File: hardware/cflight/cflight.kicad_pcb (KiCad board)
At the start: 2 copper layers, 30.5 x 81.3 mm, 13 parts, among them J1 GPS connector, J2 GPRS connector, U1 ESP32-DEVKIT-V1

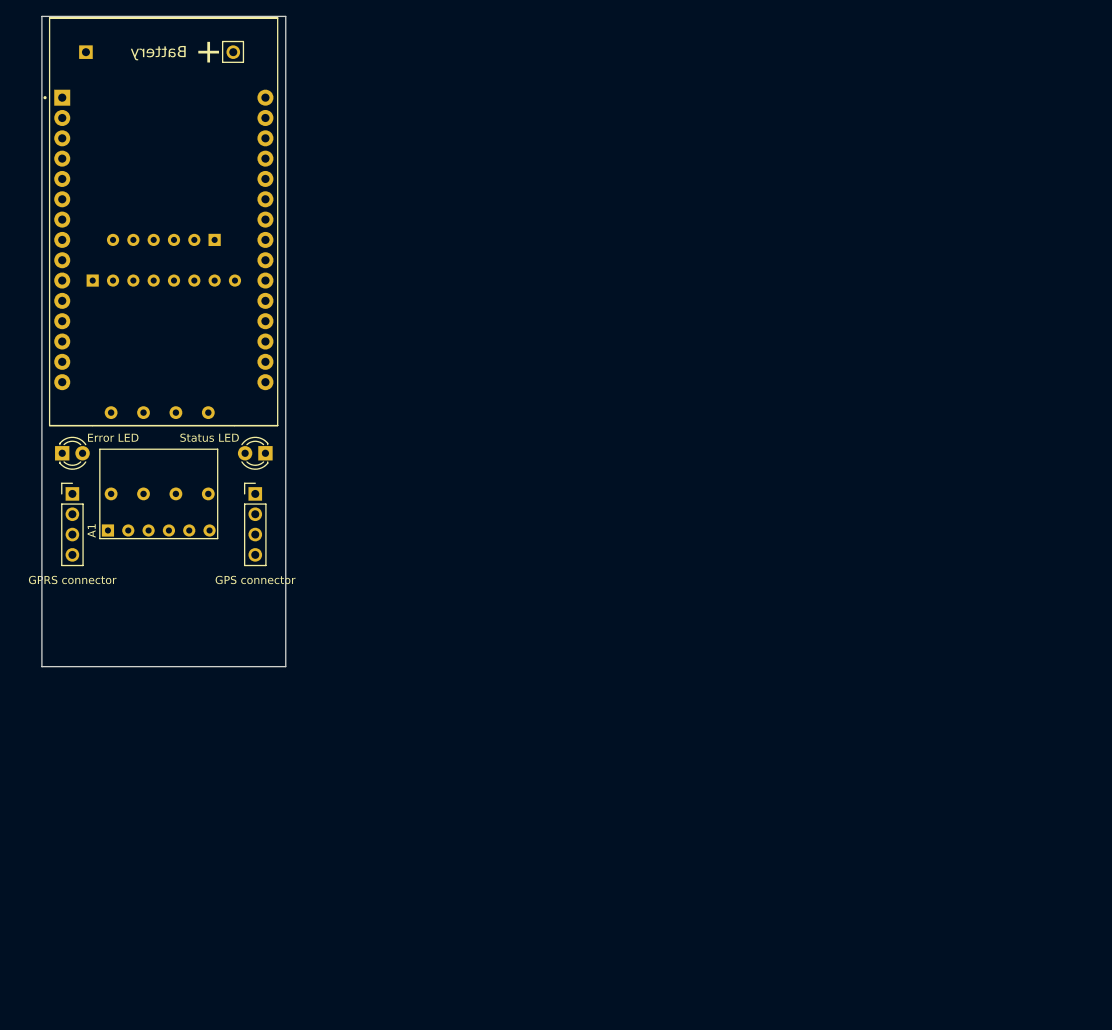
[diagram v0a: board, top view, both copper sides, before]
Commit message: college prog
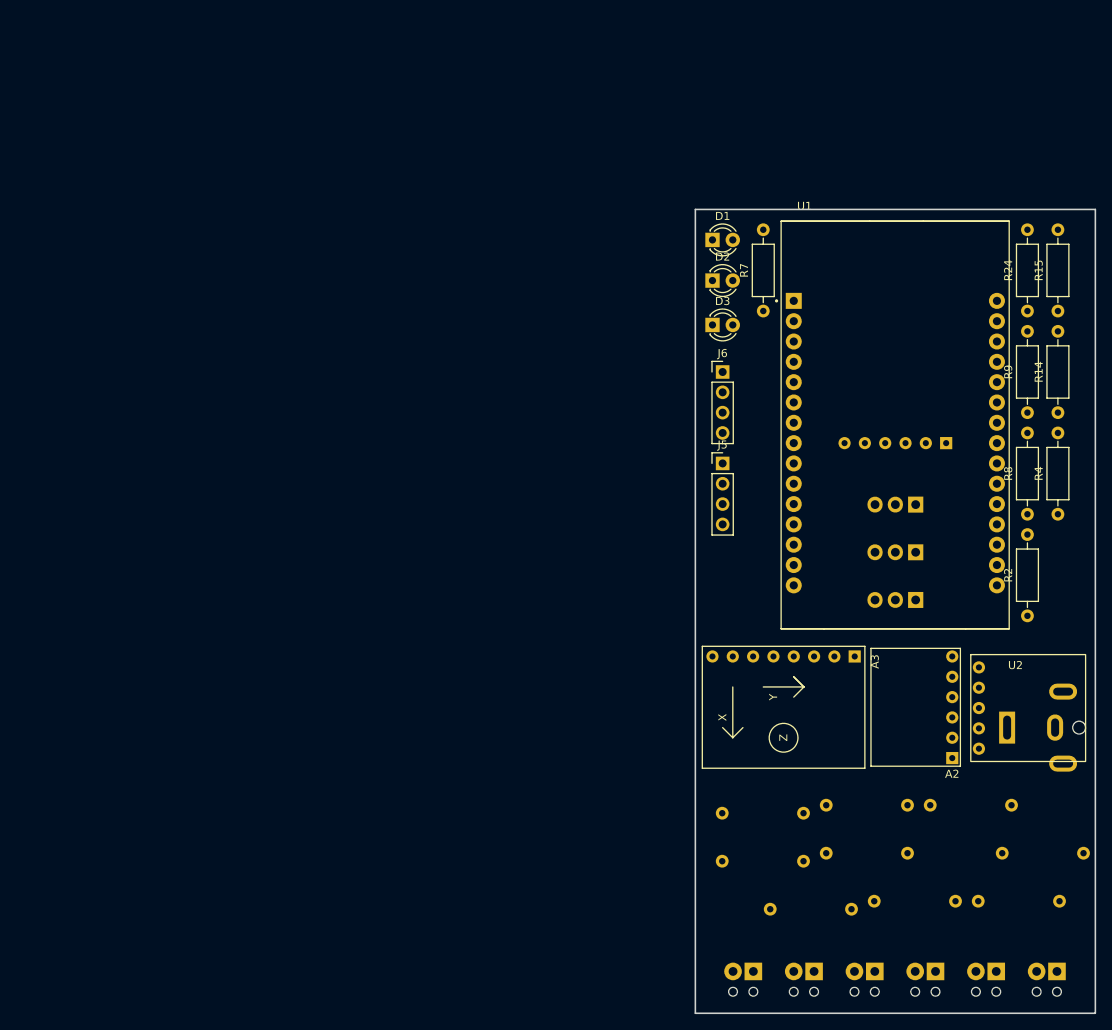
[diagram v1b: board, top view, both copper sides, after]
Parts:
- removed Battery1: Battery_Cell, Connector_PinSocket_2.54mm:PinSocket_1x02_P2.54mm_Vertical
- added D3: Status LED, LED_THT:LED_D3.0mm, F.Cu at (134.6, 64.0)
- added J10: CH_{2}, TerminalBlock_Phoenix:TerminalBlock_Phoenix_MPT-0,5-2-2.54_1x02_P2.54mm_Horizontal, B.Cu at (177.7, 144.8)
- added J3: 3.3v, TerminalBlock_Phoenix:TerminalBlock_Phoenix_MPT-0,5-2-2.54_1x02_P2.54mm_Horizontal, B.Cu at (154.9, 144.8)
- added J4: CH_{1}, TerminalBlock_Phoenix:TerminalBlock_Phoenix_MPT-0,5-2-2.54_1x02_P2.54mm_Horizontal, B.Cu at (162.5, 144.8)
- added J5: GPS connector, Connector_PinHeader_2.54mm:PinHeader_1x04_P2.54mm_Vertical, F.Cu at (135.9, 81.3)
- added J6: GPRS connector, Connector_PinHeader_2.54mm:PinHeader_1x04_P2.54mm_Vertical, F.Cu at (135.9, 69.8)
- added J7: CH_{3}, TerminalBlock_Phoenix:TerminalBlock_Phoenix_MPT-0,5-2-2.54_1x02_P2.54mm_Horizontal, B.Cu at (170.1, 144.8)
- added J8: Barrel_Jack_Switch, Connector_BarrelJack:BarrelJack_CUI_PJ-063AH_Horizontal, B.Cu at (171.4, 114.3)
- added Q1: TIP122, Package_TO_SOT_THT:TO-220-3_Vertical, B.Cu at (160.0, 86.4)
- added Q2: TIP122, Package_TO_SOT_THT:TO-220-3_Vertical, B.Cu at (160.0, 92.4)
- added Q3: TIP122, Package_TO_SOT_THT:TO-220-3_Vertical, B.Cu at (160.0, 98.3)
- added R10: 4k7, Resistor_THT:R_Axial_DIN0207_L6.3mm_D2.5mm_P10.16mm_Horizontal, B.Cu at (172.0, 124.0)
- added R11: 5k, Resistor_THT:R_Axial_DIN0207_L6.3mm_D2.5mm_P10.16mm_Horizontal, B.Cu at (146.0, 131.0)
- added R12: 10k, Resistor_THT:R_Axial_DIN0207_L6.3mm_D2.5mm_P10.16mm_Horizontal, B.Cu at (152.0, 137.0)
- added R13: 4k7, Resistor_THT:R_Axial_DIN0207_L6.3mm_D2.5mm_P10.16mm_Horizontal, B.Cu at (159.0, 124.0)
- added R14: 470, Resistor_THT:R_Axial_DIN0207_L6.3mm_D2.5mm_P10.16mm_Horizontal, F.Cu at (177.8, 74.9)
- added R15: 80, Resistor_THT:R_Axial_DIN0207_L6.3mm_D2.5mm_P10.16mm_Horizontal, F.Cu at (177.8, 62.2)
- added R23: 4k7, Resistor_THT:R_Axial_DIN0207_L6.3mm_D2.5mm_P10.16mm_Horizontal, B.Cu at (159.0, 130.0)
- added R24: 470, Resistor_THT:R_Axial_DIN0207_L6.3mm_D2.5mm_P10.16mm_Horizontal, F.Cu at (174.0, 62.2)
- added R5: 12k, Resistor_THT:R_Axial_DIN0207_L6.3mm_D2.5mm_P10.16mm_Horizontal, B.Cu at (165.0, 136.0)
- added R6: 10k, Resistor_THT:R_Axial_DIN0207_L6.3mm_D2.5mm_P10.16mm_Horizontal, B.Cu at (181.0, 130.0)
- added R7: 80, Resistor_THT:R_Axial_DIN0207_L6.3mm_D2.5mm_P10.16mm_Horizontal, F.Cu at (141.0, 62.2)
- added R8: 470, Resistor_THT:R_Axial_DIN0207_L6.3mm_D2.5mm_P10.16mm_Horizontal, F.Cu at (174.0, 87.6)
- added R9: 50, Resistor_THT:R_Axial_DIN0207_L6.3mm_D2.5mm_P10.16mm_Horizontal, F.Cu at (174.0, 74.9)
- added U2: ~, Modules:GY-271, F.Cu at (166.9, 105.2)
- A1: value BMP280_Module -> SD_Card_Module; footprint Modules:BMP280_Module -> Modules:SD_Card_Module; moved to B.Cu
- A2: value SD_Card_Module -> BMP280_Module; footprint Modules:SD_Card_Module -> Modules:BMP280_Module; moved to F.Cu
- A3: moved to F.Cu
- D1: value Error LED -> Arm LED
- D2: value Status LED -> Error LED
- J1: value GPS connector -> 7.2v; footprint Connector_PinHeader_2.54mm:PinHeader_1x04_P2.54mm_Vertical -> TerminalBlock_Phoenix:TerminalBlock_Phoenix_MPT-0,5-2-2.54_1x02_P2.54mm_Horizontal; moved to B.Cu
- J2: value GPRS connector -> I2C; footprint Connector_PinHeader_2.54mm:PinHeader_1x04_P2.54mm_Vertical -> TerminalBlock_Phoenix:TerminalBlock_Phoenix_MPT-0,5-2-2.54_1x02_P2.54mm_Horizontal; moved to B.Cu
- R1: value 80 -> 10k
- R2: value 50 -> 18k; moved to F.Cu
- R3: value 1800 -> 5k
- R4: value 1200 -> 5k; moved to F.Cu
- moved R1 129.0 mm to (178.0, 136.0), turned to 180 degrees
- moved A2 112.7 mm to (164.6, 118.1), turned to 180 degrees
- moved R2 111.5 mm to (174.0, 100.3)
- moved J2 110.3 mm to (147.3, 144.8), turned to 180 degrees
- moved R4 106.2 mm to (177.8, 87.6)
- moved A3 106.2 mm to (152.4, 105.4)
- moved A1 105.3 mm to (163.8, 78.7)
- moved U1 94.9 mm to (157.5, 76.5)
- moved R3 88.0 mm to (146.0, 125.0), turned to 180 degrees
- moved J1 86.3 mm to (139.7, 144.8), turned to 180 degrees
- moved D1 85.5 mm to (134.6, 53.3)
- moved D2 59.9 mm to (134.6, 58.4), turned to 0 degrees
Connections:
- A1 pad 2: Batt_{gnd} -> SPI_{CS}
- A1 pad 3: SCL -> MOSI
- A1 pad 4: SDA -> SPI_{CLK}
- A1 pad 5: unconnected-(A1-CSB-Pad5) -> MISO
- A1 pad 6: unconnected-(A1-SD0-Pad6) -> Batt_{gnd}
- A2 pad 2: SPI_{CS} -> Batt_{gnd}
- A2 pad 3: MOSI -> SCL
- A2 pad 4: SPI_{CLK} -> SDA
- A2 pad 5: MISO -> unconnected-(A2-CSB-Pad5)
- A2 pad 6: Batt_{gnd} -> unconnected-(A2-SD0-Pad6)
- A3 pad 1: unconnected-(A3-VCC-Pad1) -> +3.3V
- J1 pad 1: +3.3V -> V_{batt}
- J2 pad 1: +3.3V -> SCL
- J2 pad 2: Batt_{gnd} -> SDA
- R1 pad 1: Net-(D1-A) -> CH_{1}^{test}
- R1 pad 2: LED_{status} -> Net-(J4-Pin_2)
- R2 pad 1: Net-(D2-A) -> V_{batt}
- R2 pad 2: LED_{error} -> BATT_{check}
- R3 pad 1: V_{batt} -> Batt_{gnd}
- R3 pad 2: BATT_{check} -> CH_{1}^{test}
- R4 pad 2: BATT_{check} -> CH_{2}^{test}
- U1 pad 19: unconnected-(U1-D34-Pad19) -> CH_{2}^{test}
- U1 pad 20: unconnected-(U1-D35-Pad20) -> CH_{2}^{fire}
- U1 pad 21: unconnected-(U1-D32-Pad21) -> CH_{1}^{fire}
- U1 pad 22: unconnected-(U1-D33-Pad22) -> CH_{1}^{test}
- U1 pad 27: unconnected-(U1-D12-Pad27) -> CH_{3}^{test}
- U1 pad 28: unconnected-(U1-D13-Pad28) -> CH_{3}^{fire}
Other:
- board size 30.5 x 81.3 mm -> 50 x 100.5 mm
- board text removed: "Battery"

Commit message: Continue hardware
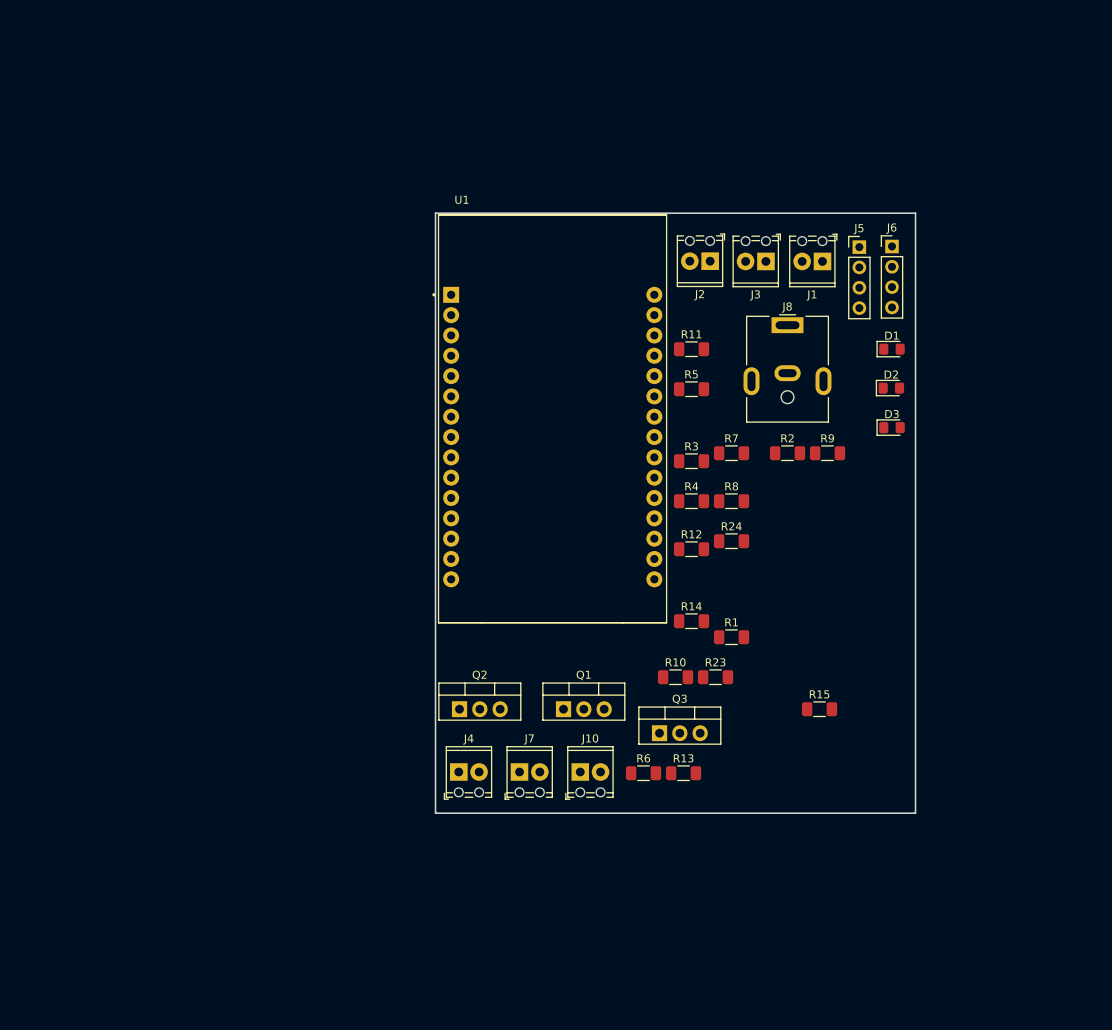
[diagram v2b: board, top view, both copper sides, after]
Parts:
- removed A1: SD_Card_Module, Modules:SD_Card_Module
- removed A2: BMP280_Module, Modules:BMP280_Module
- removed A3: MPU6050, Modules:MPU6050_Module
- removed U2: ~, Modules:GY-271
- D1: value Arm LED -> Armed; footprint LED_THT:LED_D3.0mm -> LED_SMD:LED_0805_2012Metric_Pad1.15x1.40mm_HandSolder
- D2: value Error LED -> Error; footprint LED_THT:LED_D3.0mm -> LED_SMD:LED_0805_2012Metric_Pad1.15x1.40mm_HandSolder
- D3: value Status LED -> Status; footprint LED_THT:LED_D3.0mm -> LED_SMD:LED_0805_2012Metric_Pad1.15x1.40mm_HandSolder
- J1, J10, J2, J3, J4, J7, J8, Q1, Q2, Q3: moved to F.Cu
- J5: value GPS connector -> GPS
- J6: value GPRS connector -> GPRS
- R1, R10, R11, R12, R13, R23, R3, R5, R6: footprint Resistor_THT:R_Axial_DIN0207_L6.3mm_D2.5mm_P10.16mm_Horizontal -> Resistor_SMD:R_1206_3216Metric_Pad1.30x1.75mm_HandSolder; moved to F.Cu
- R14, R15, R2, R24, R4, R7, R8, R9: footprint Resistor_THT:R_Axial_DIN0207_L6.3mm_D2.5mm_P10.16mm_Horizontal -> Resistor_SMD:R_1206_3216Metric_Pad1.30x1.75mm_HandSolder
- moved J3 89.8 mm to (141.3, 56.0)
- moved J2 89.7 mm to (134.3, 56.0)
- moved J1 89.2 mm to (148.4, 56.0)
- moved R5 72.0 mm to (132.0, 72.0), turned to 0 degrees
- moved R11 65.5 mm to (132.0, 67.0), turned to 0 degrees
- moved J10 64.6 mm to (118.1, 119.8), turned to 0 degrees
- moved J4 64.6 mm to (102.9, 119.8), turned to 0 degrees
- moved J7 64.6 mm to (110.5, 119.8), turned to 0 degrees
- moved Q2 60.3 mm to (103.0, 112.0), turned to 0 degrees
- moved R15 58.0 mm to (148.0, 112.0), turned to 0 degrees
- moved J8 57.3 mm to (144.0, 64.0), turned to 0 degrees
- moved R6 55.9 mm to (126.0, 120.0), turned to 0 degrees
- moved R14 52.7 mm to (132.0, 101.0), turned to 0 degrees
- moved R1 52.6 mm to (137.0, 103.0), turned to 0 degrees
- moved Q1 50.9 mm to (116.0, 112.0), turned to 0 degrees
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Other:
- board size 50 x 100.5 mm -> 60 x 75 mm
